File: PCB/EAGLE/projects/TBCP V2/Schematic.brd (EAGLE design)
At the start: 160 x 71.1 mm, 110 parts, among them J1 12 Supply, J2 TB Header, J3 FP Header, Q1 DMP4025LK3Q-13, U1 ESP32-DEVKITC, U100 ADS1115, U101 TLE9201SG, U2 7805

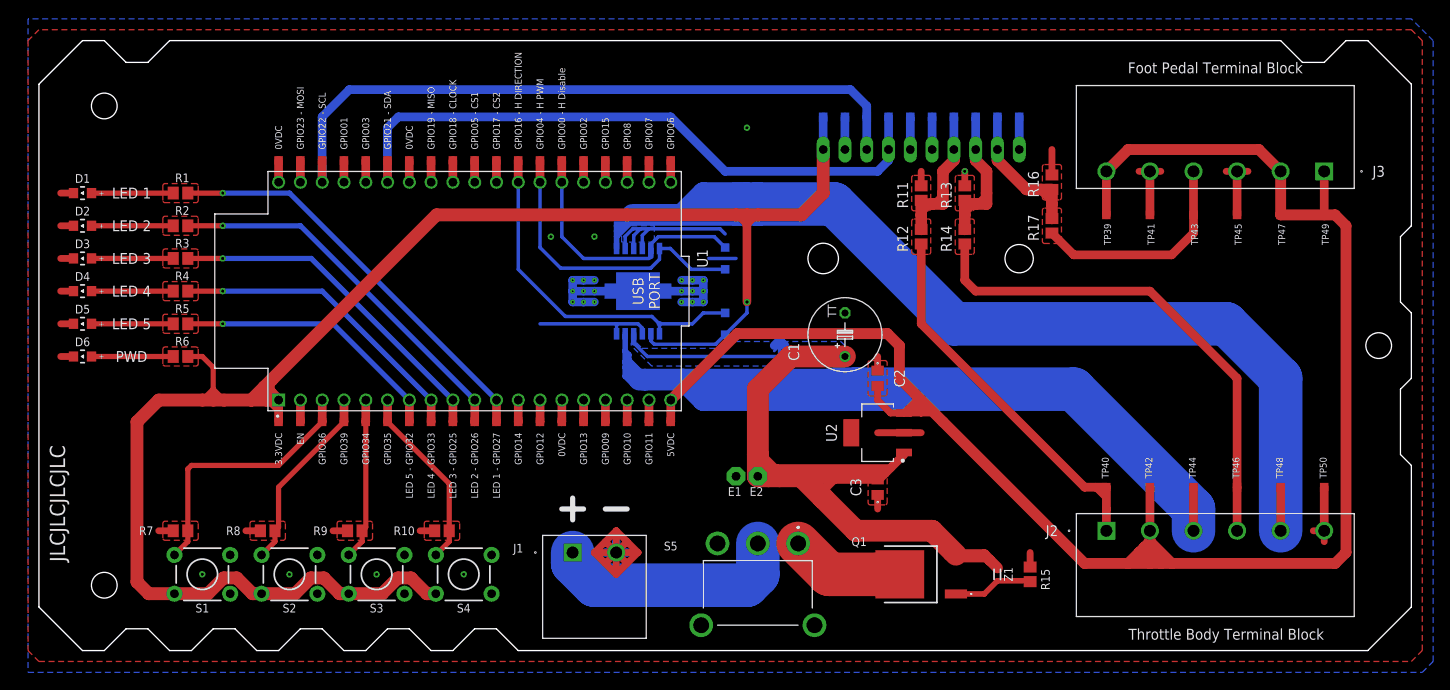
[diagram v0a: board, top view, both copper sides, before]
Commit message: Added A1 PDF
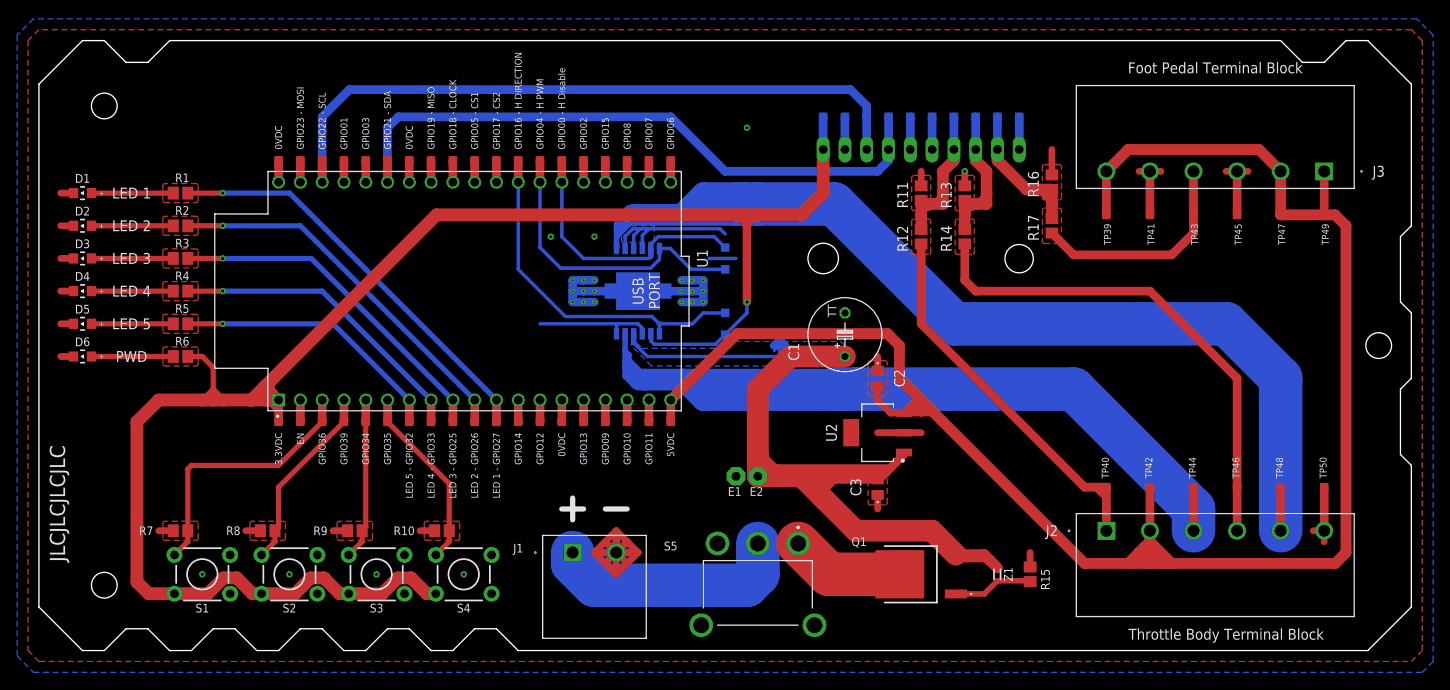
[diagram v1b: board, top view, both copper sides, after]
